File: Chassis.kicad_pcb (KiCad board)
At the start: 2 copper layers, 125.5 x 120 mm, 47 parts, among them IC1 RT6285GSP, IC2 LV2862YDDCR, J1 FR_JST, J10 BL_XT30, J11 Sabre Vertical Header 6, J12 Conn_01x12, J2 FR_XT30, J3 BR_JST, J4 BR_XT30, J5 IN_JST, J6 IN_XT60, J7 FL_JST, J8 FL_XT30, J9 BL_JST

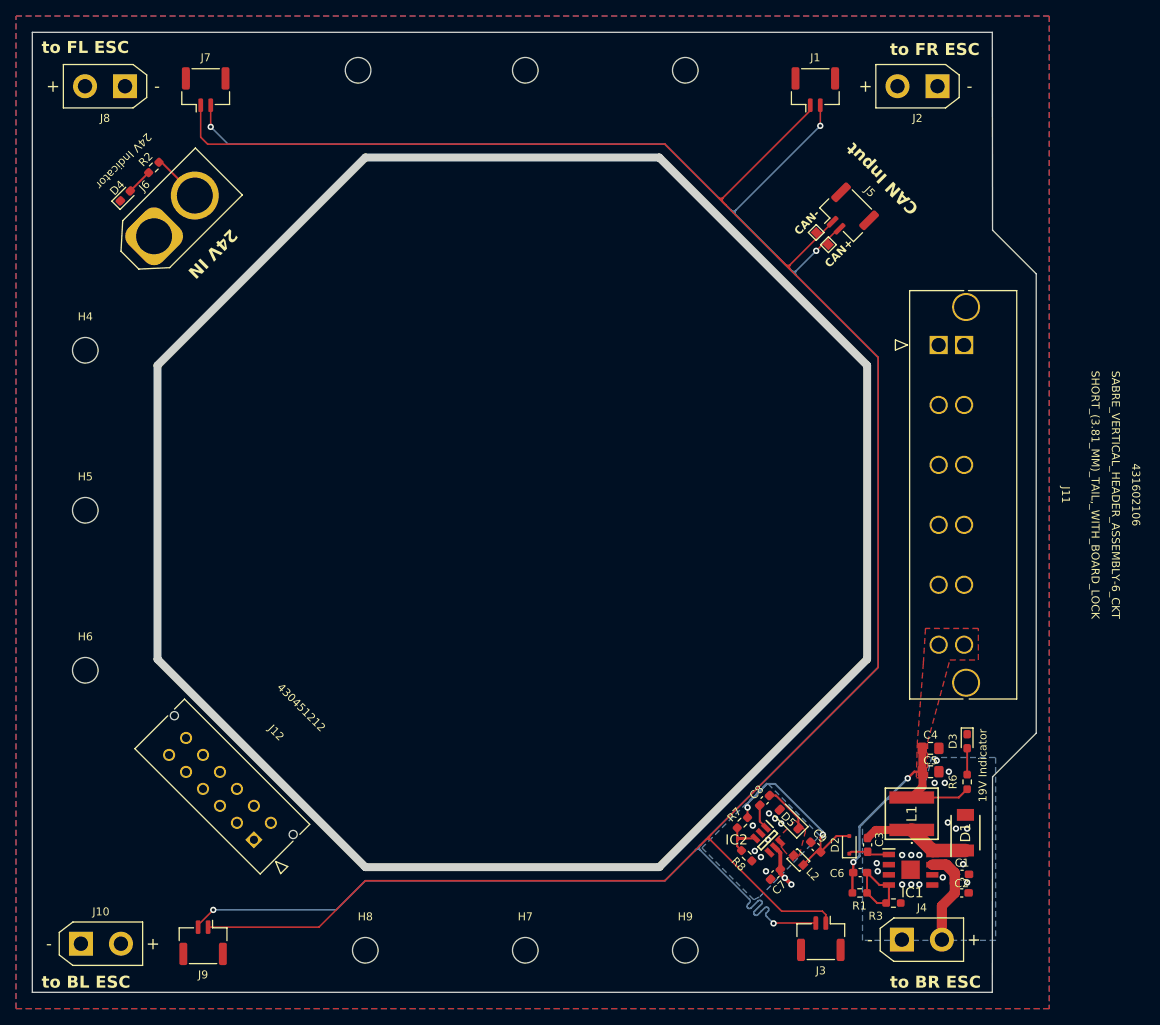
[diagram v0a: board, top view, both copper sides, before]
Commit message: U
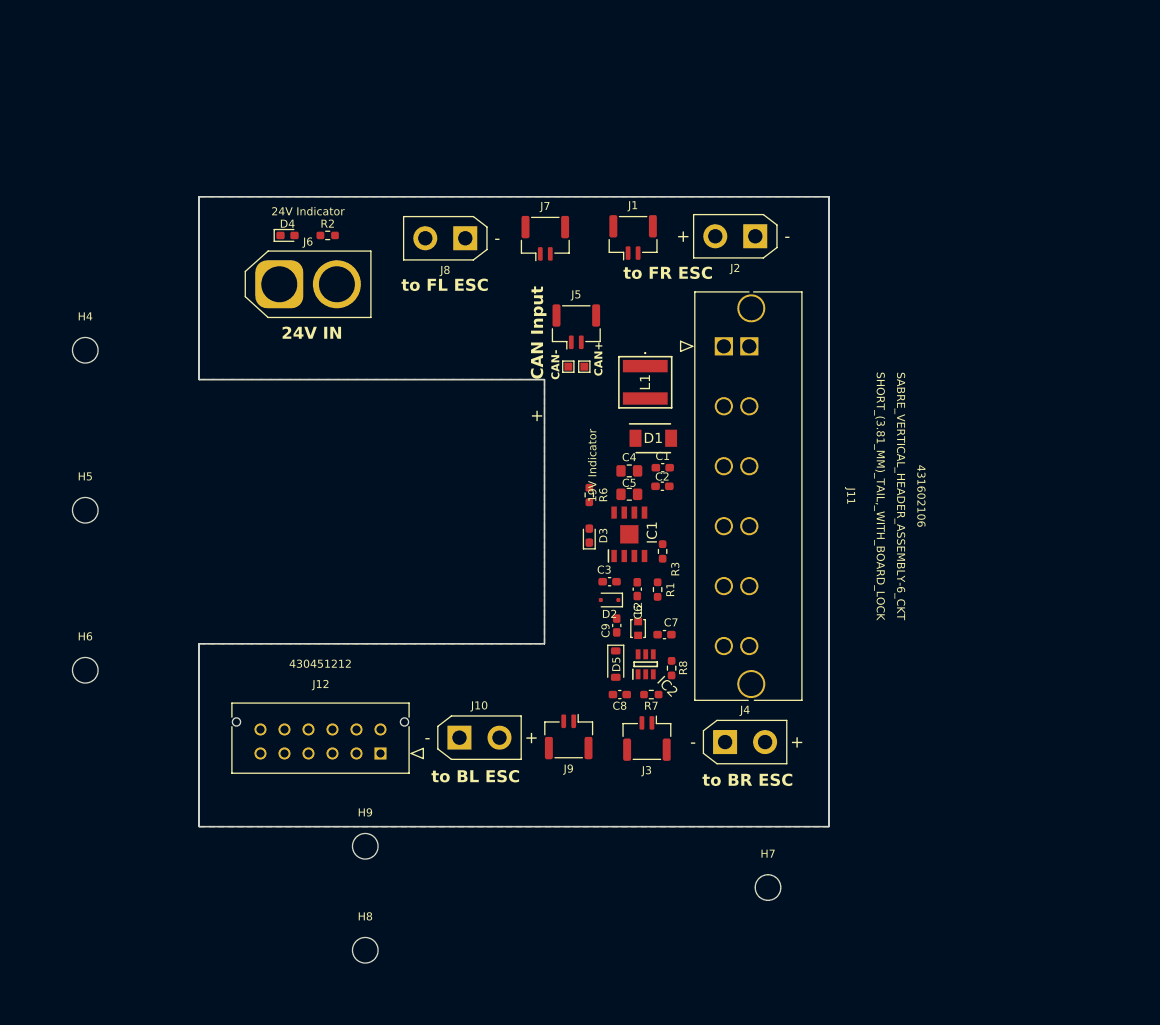
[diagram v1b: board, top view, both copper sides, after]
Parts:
- removed H1, H2, H3: MountingHole, MountingHole:MountingHole_3.2mm_M3
- moved L1 63.4 mm to (165.0, 74.0), turned to -90 degrees
- moved C2 63.1 mm to (167.1, 87.0)
- moved C1 63.1 mm to (167.2, 84.7)
- moved D1 62.9 mm to (166.0, 81.0), turned to 0 degrees
- moved R6 59.3 mm to (158.0, 88.1), turned to -90 degrees
- moved IC1 54.7 mm to (163.0, 93.0), turned to 90 degrees
- moved J10 53.9 mm to (141.8, 118.4)
- moved D3 53.8 mm to (158.0, 93.2), turned to 90 degrees
- moved R3 52.6 mm to (167.2, 95.1), turned to 90 degrees
- moved J9 52.4 mm to (155.4, 118.3)
- moved C4 51.2 mm to (163.0, 85.1)
- moved C5 51.2 mm to (163.0, 88.0)
- moved J8 46.6 mm to (142.5, 56.0)
- moved J7 46.3 mm to (152.5, 56.0)
- moved C3 46.1 mm to (160.5, 98.9), turned to 180 degrees
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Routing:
- net /CAN+: track 299.6 -> 0.00 mm, vias 5 -> 0
- net /CAN-: track 286.8 -> 0.00 mm
- net /V_{OUT}: track 33.4 -> 0.00 mm, vias 2 -> 0
- net +24V: track 28.5 -> 0.00 mm, vias 2 -> 0
- net +5V: track 24.6 -> 0.00 mm, vias 2 -> 0
- net /24V -> 19V Buck Convertor/SW_{19}: track 13.7 -> 0.00 mm
- net /24V -> 19V Buck Convertor/FB_{19}: track 11.2 -> 0.00 mm
- net /24V -> 19V Buck Convertor/FB_{5}: track 7.42 -> 0.00 mm
- net /24V -> 19V Buck Convertor/SW_{5}: track 6.08 -> 0.00 mm
- net /24V -> 19V Buck Convertor/BOOT_{19}: track 5.19 -> 0.00 mm
- net Net-(D3-A): track 3.29 -> 0.00 mm
- net Net-(D4-A): track 3.24 -> 0.00 mm
- net /24V -> 19V Buck Convertor/BOOT_{5}: track 3.13 -> 0.00 mm
- net GND: track 0.21 -> 0.00 mm, vias 26 -> 0
- removed copper zone on B.Cu, net +24V
- removed copper zone on F.Cu, net /24V -> 19V Buck Convertor/FB_{19}
- removed copper zone on F.Cu, net /24V -> 19V Buck Convertor/SW_{5}
- removed copper zone on F.Cu, net /V_{OUT}
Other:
- board size 125.5 x 120 mm -> 78.7 x 94.5 mm
